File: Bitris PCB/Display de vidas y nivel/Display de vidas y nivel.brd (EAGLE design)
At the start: 41.6 x 29.2 mm, 7 parts, among them T1 BC848, T2 BC848

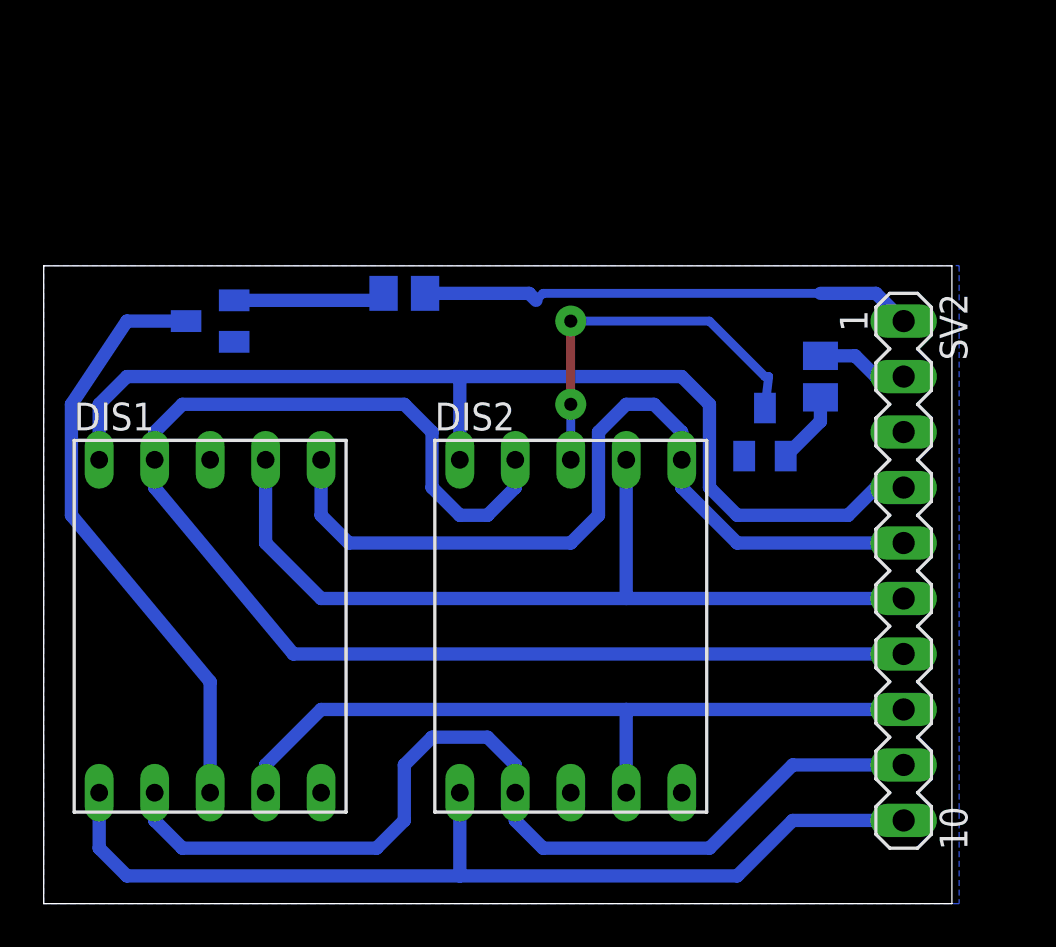
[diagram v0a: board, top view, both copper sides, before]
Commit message: PCB DISPLAYs
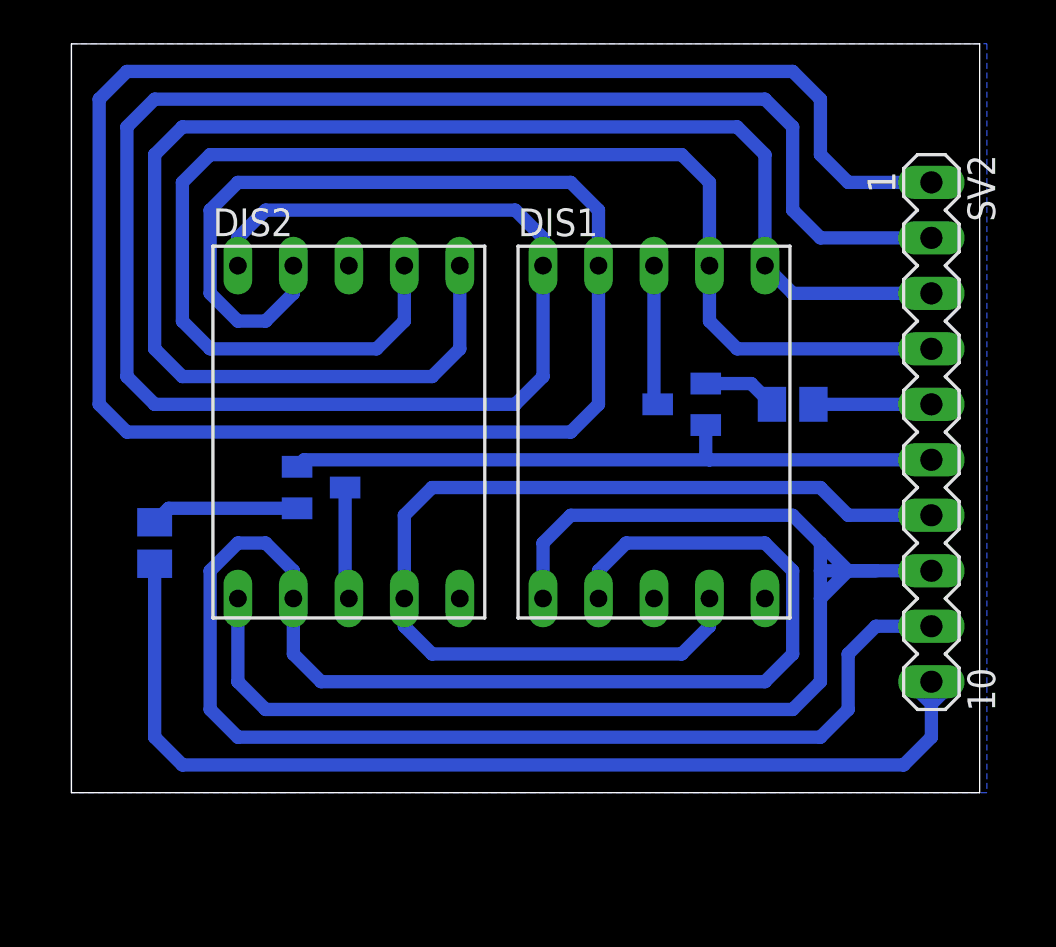
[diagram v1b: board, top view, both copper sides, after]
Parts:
- moved R4 31.4 mm to (16.5, 36.8), turned to 90 degrees
- moved DIS1 22.2 mm to (39.4, 41.9)
- moved T1 21.9 mm to (40.6, 43.2)
- moved T2 20.5 mm to (24.1, 39.4), turned to 90 degrees
- moved R3 18.5 mm to (45.7, 43.2)
- moved DIS2 13.5 mm to (25.4, 41.9)
- moved SV2 6.48 mm to (52.1, 41.9)
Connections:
- removed net N$11: R4.1, SV2.2
- new net N$17: R4.1, SV2.10
- net GND: now also SV2.6; no longer SV2.3
- net N$10: now also SV2.5; no longer SV2.1
- net N$13: now also SV2.4; no longer SV2.6
- net N$2: now also SV2.3; no longer SV2.5
- net N$3: now also SV2.7; no longer SV2.8
- net N$5: now also SV2.8; no longer SV2.10
- net N$6: now also SV2.1; no longer SV2.7
- net N$7: now also SV2.2; no longer SV2.4
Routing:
- net N$6: track 62.8 -> 117.8 mm
- net N$17: track 0.00 -> 50.7 mm
- net N$7: track 49.1 -> 96.4 mm
- net N$4: track 44.8 -> 91.1 mm
- net N$2: track 38.7 -> 69.9 mm
- net GND: track 0.00 -> 30.8 mm
- net N$13: track 40.4 -> 62.3 mm
- net N$8: track 27.4 -> 6.59 mm
- net N$5: track 44.8 -> 62.8 mm
- net N$10: track 22.7 -> 5.40 mm
- net N$9: track 17.9 -> 5.15 mm, vias 2 -> 0
- net N$3: track 35.3 -> 46.6 mm
- net N$11: track 4.66 -> 0.00 mm
- net N$1: track 6.97 -> 3.42 mm
- net N$12: track 3.35 -> 6.79 mm
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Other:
- board size 41.6 x 29.2 mm -> 41.6 x 34.3 mm
